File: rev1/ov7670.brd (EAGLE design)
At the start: 60.3 x 44.4 mm, 3 parts

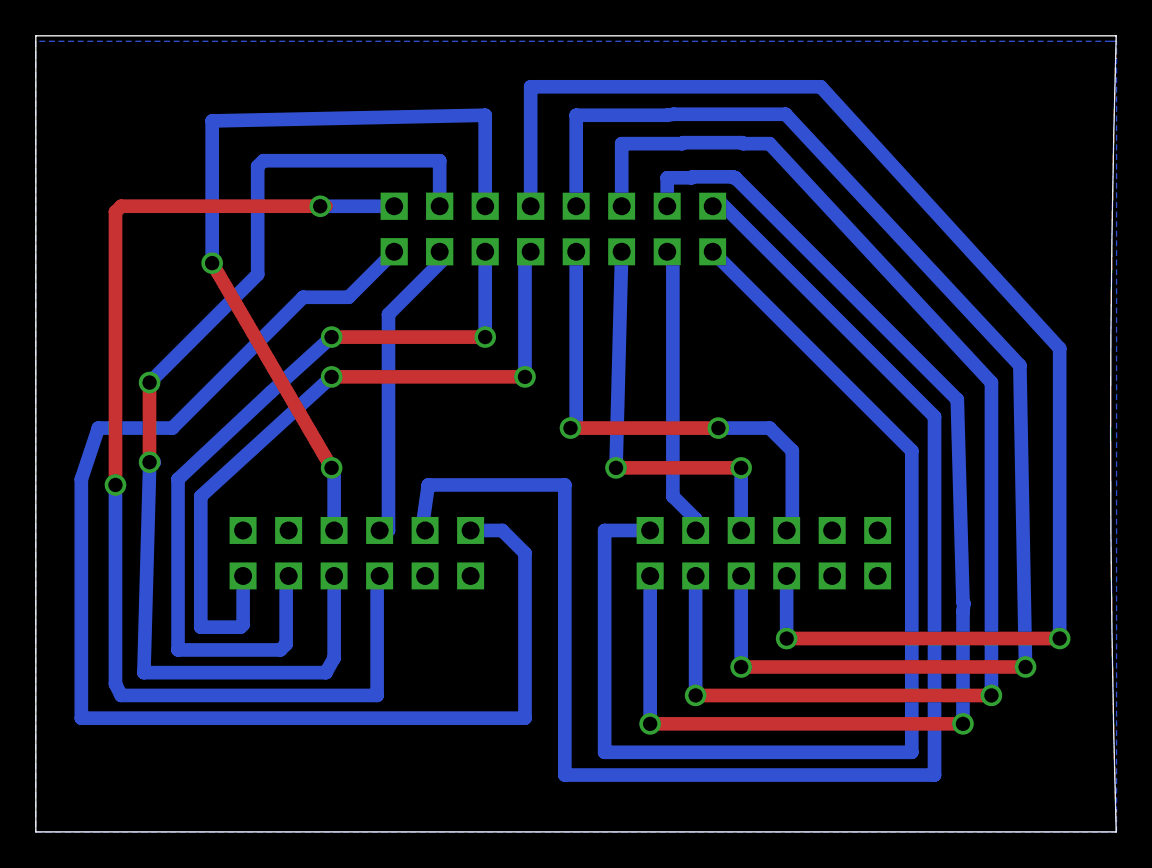
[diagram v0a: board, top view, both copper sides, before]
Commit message: update to rev2
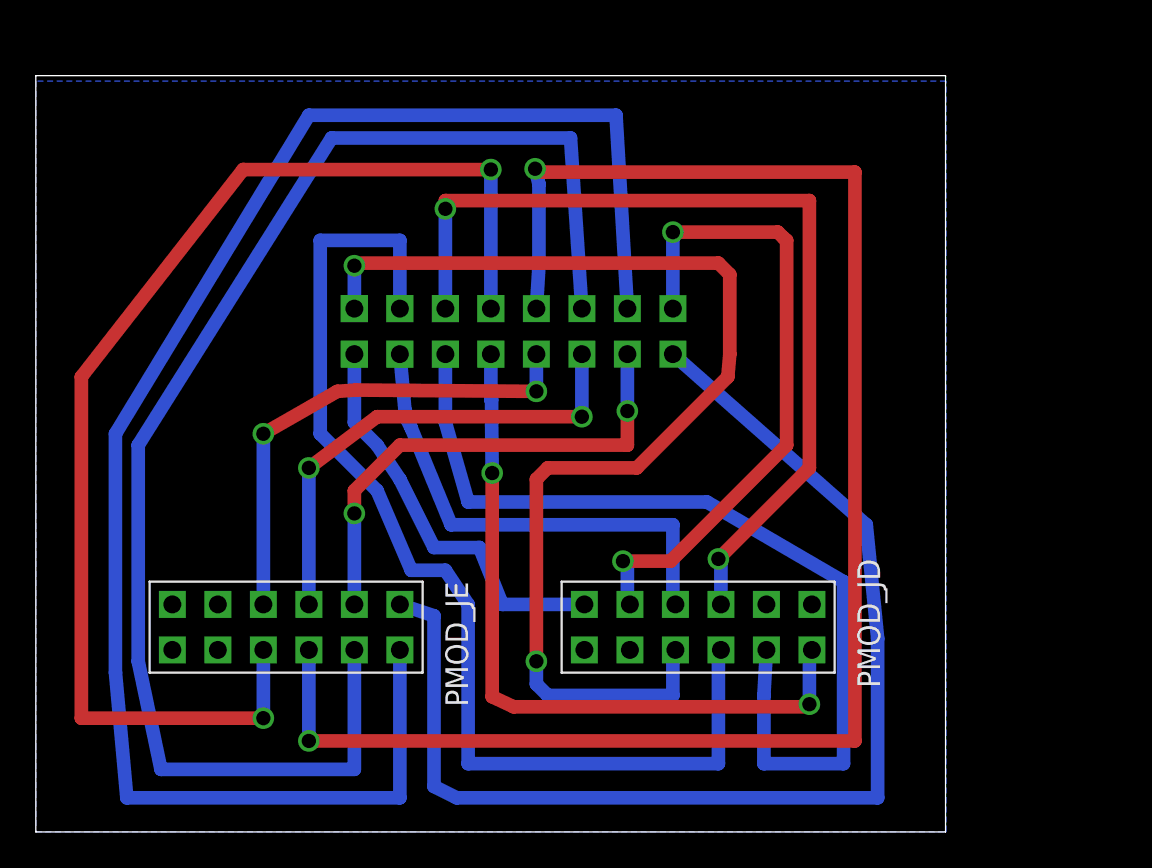
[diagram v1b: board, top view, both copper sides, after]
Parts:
- moved U$3 27.0 mm to (14.0, 12.7), flipped to the top
- moved U$2 19.5 mm to (37.0, 8.89), flipped to the top
- moved U$1 6.13 mm to (25.4, 29.2)
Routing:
- net 3V3: track 74.5 -> 22.7 mm
- net GND: track 84.6 -> 36.8 mm, vias 0 -> 2
- net D6: track 66.8 -> 92.6 mm, vias 2 -> 0
- net D2: track 73.7 -> 93.0 mm
- net D5: track 16.2 -> 27.7 mm, vias 0 -> 2
- net VSYNC: track 17.5 -> 27.3 mm
- net D0: track 77.6 -> 69.3 mm
- net D4: track 70.6 -> 78.8 mm, vias 2 -> 0
- net XCLK: track 44.6 -> 51.5 mm, vias 2 -> 0
- net SCL: track 45.0 -> 51.1 mm
- net D3: track 22.5 -> 27.3 mm
- net PLCK: track 59.7 -> 61.9 mm, vias 2 -> 0
- net D7: track 64.6 -> 66.1 mm
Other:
- board size 60.3 x 44.4 mm -> 50.8 x 42.2 mm
